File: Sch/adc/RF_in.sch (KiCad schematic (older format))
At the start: 73 parts, among them CN1 SMA, CN2 SMA, J3 JP2, J4 JP2, J5 JP2, U1 LTC2292, U2 BGA2818, U4 BGA2818, U5 CDCLVC1102, X1 ECS-TXO-2520

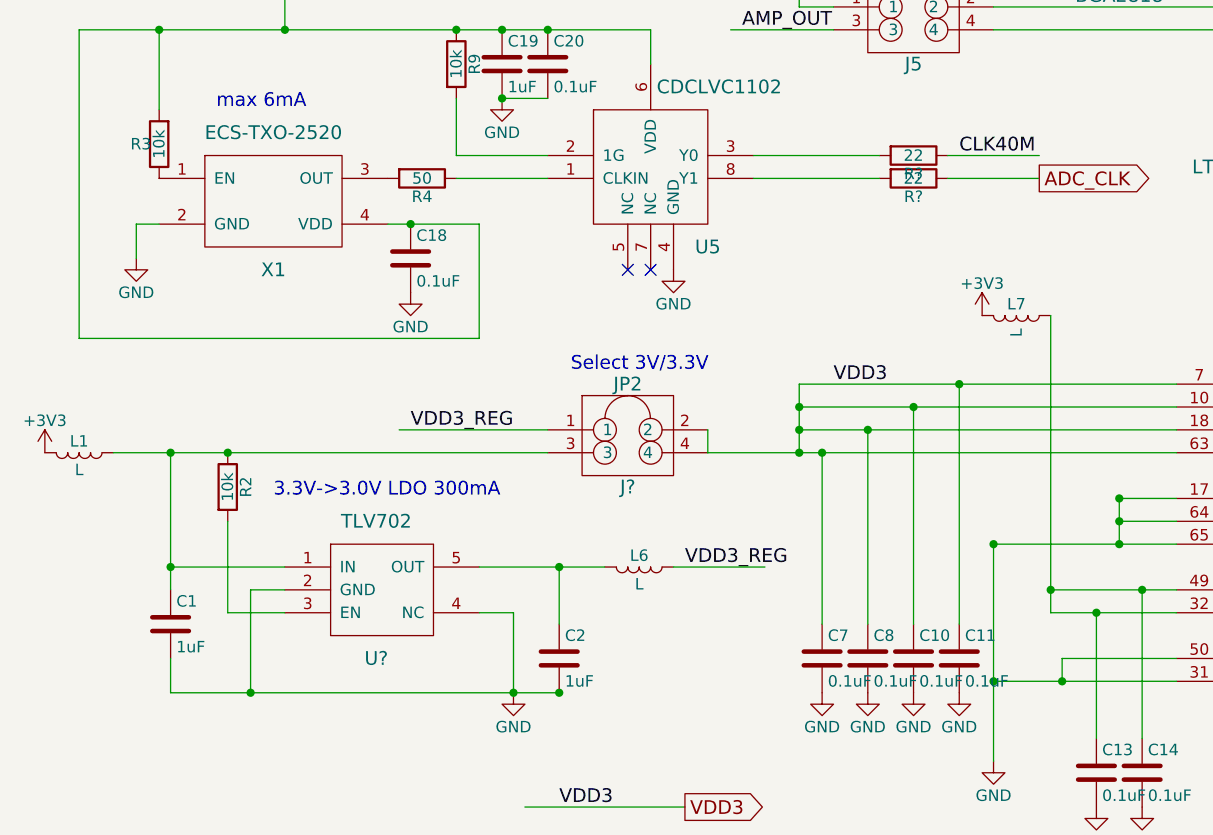
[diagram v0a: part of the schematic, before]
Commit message: Schematics done
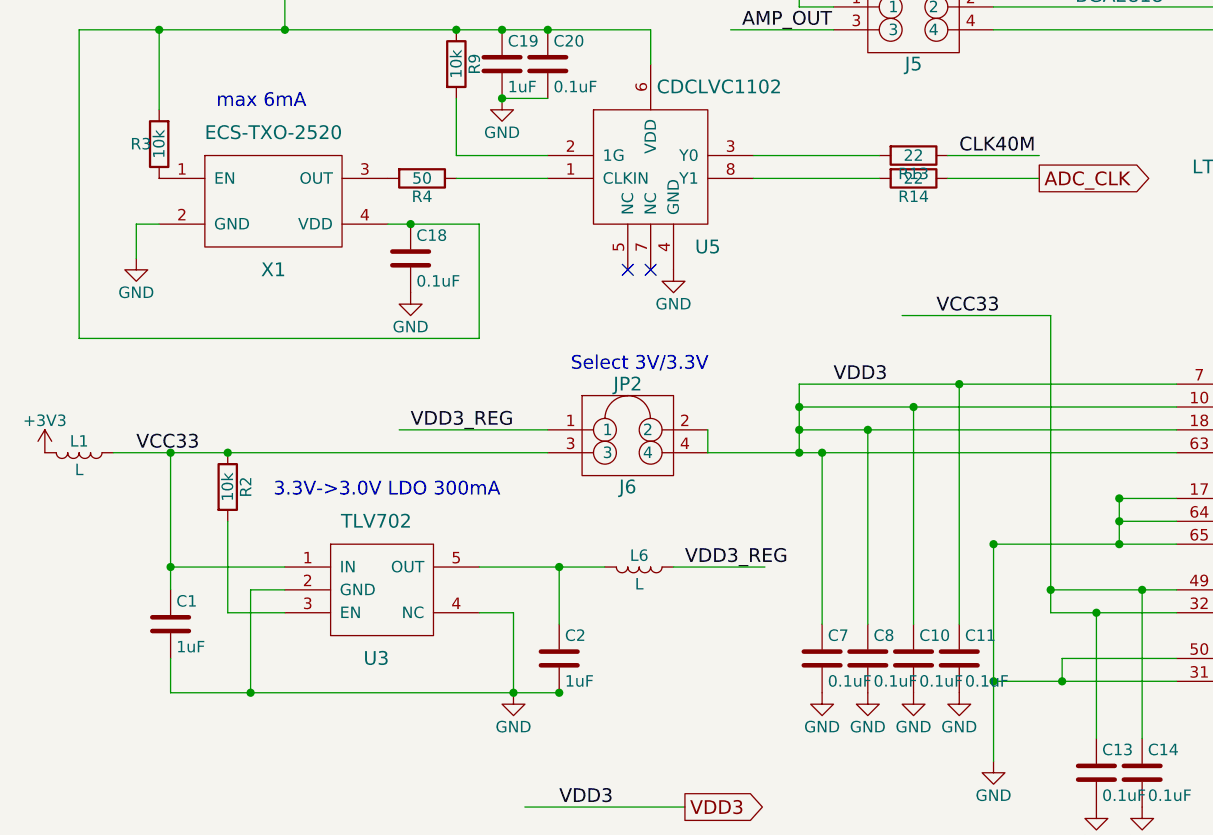
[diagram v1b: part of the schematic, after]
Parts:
- removed L7: L, symbol L
- gave numbers to parts that had none: 4
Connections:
- net labels added: VCC33
- wire segments 141 -> 142
